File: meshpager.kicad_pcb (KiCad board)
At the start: 4 copper layers, 90 x 64 mm, 14 parts, among them J3 009155003301006, J4 USB_C_Receptacle_USB2.0_16P, J5 S8B-PH-SM4-TB, U1 RAK4630-8-SM-I

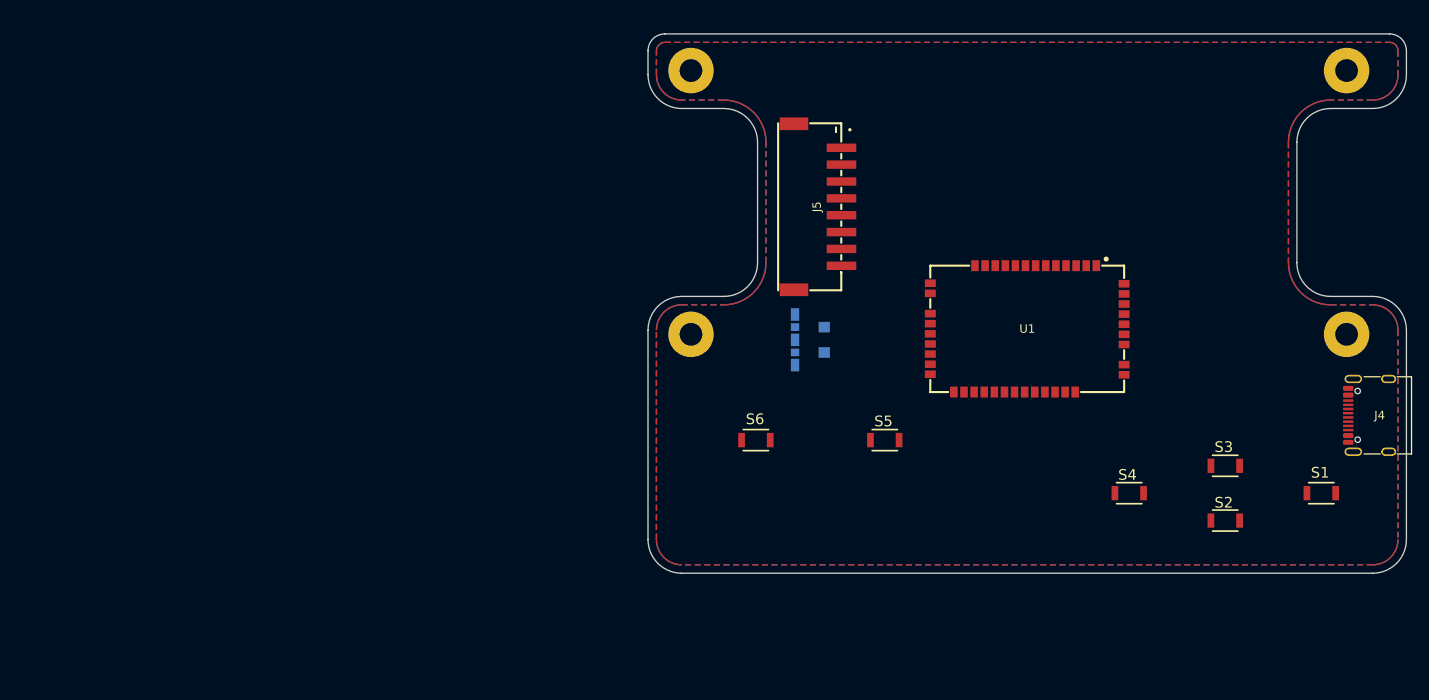
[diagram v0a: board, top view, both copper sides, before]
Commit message: Update
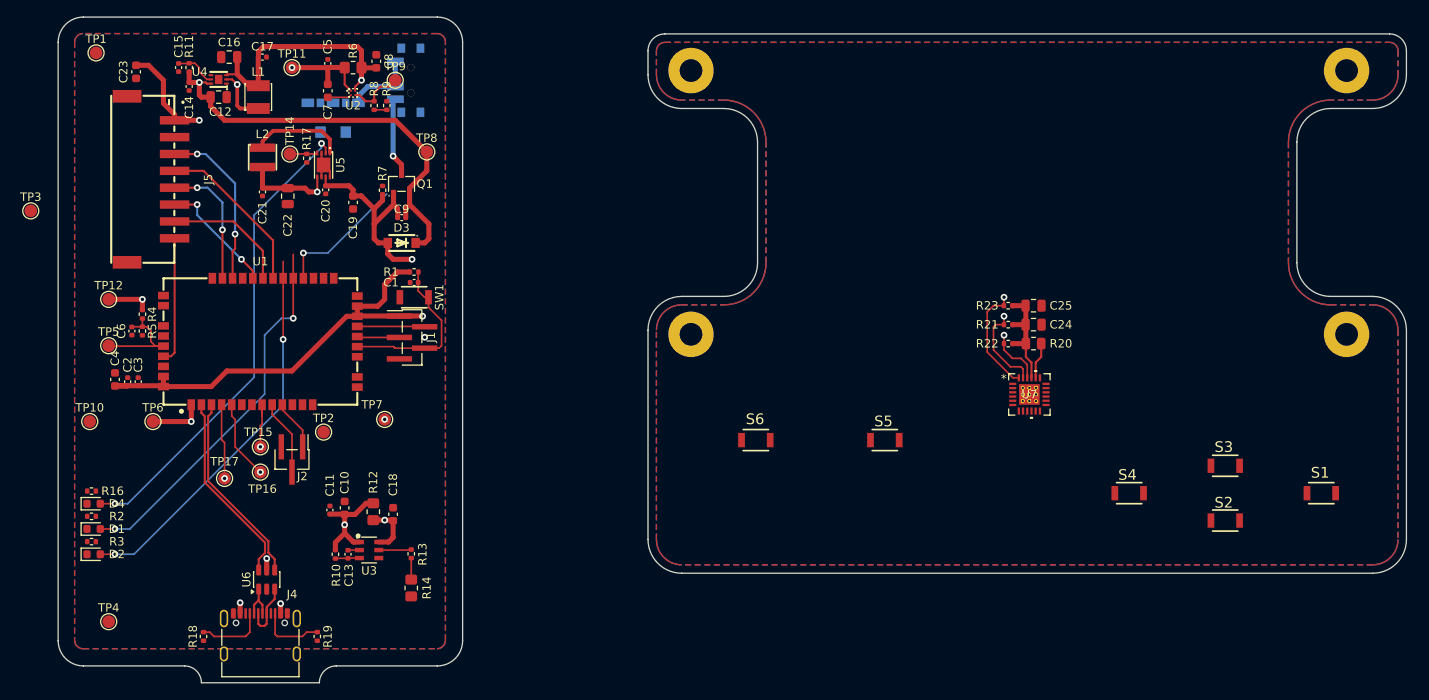
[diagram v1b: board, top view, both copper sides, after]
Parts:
- added C1: 100nF, Capacitor_SMD:C_0402_1005Metric, F.Cu at (72.2, 79.5)
- added C10: 10uF, Capacitor_SMD:C_0603_1608Metric, F.Cu at (64.0, 106.2)
- added C11: 100nF, Capacitor_SMD:C_0402_1005Metric, F.Cu at (62.2, 106.5)
- added C12: 22uF, Capacitor_SMD:C_0805_2012Metric, F.Cu at (49.0, 57.5)
- added C13: 100nF, Capacitor_SMD:C_0402_1005Metric, F.Cu at (64.4, 111.8)
- added C14: 100nF, Capacitor_SMD:C_0402_1005Metric, F.Cu at (45.5, 56.2)
- added C15: 100nF, Capacitor_SMD:C_0402_1005Metric, F.Cu at (44.3, 54.0)
- added C16: 22uF, Capacitor_SMD:C_0805_2012Metric, F.Cu at (50.3, 52.8)
- added C17: 100nF, Capacitor_SMD:C_0402_1005Metric, F.Cu at (54.2, 52.8)
- added C18: 10uF, Capacitor_SMD:C_0603_1608Metric, F.Cu at (69.8, 107.0)
- added C19: 10uF, Capacitor_SMD:C_0603_1608Metric, F.Cu at (65.0, 70.0)
- added C2: 100nF, Capacitor_SMD:C_0402_1005Metric, F.Cu at (38.2, 91.3)
- added C20: 100nF, Capacitor_SMD:C_0402_1005Metric, F.Cu at (61.8, 68.5)
- added C21: 100nF, Capacitor_SMD:C_0402_1005Metric, F.Cu at (54.2, 68.8)
- added C22: 22uF, Capacitor_SMD:C_0805_2012Metric, F.Cu at (57.2, 69.2)
- added C23: 10uF, Capacitor_SMD:C_0603_1608Metric, F.Cu at (39.2, 54.5)
- added C24: 100nF, Capacitor_SMD:C_0805_2012Metric, F.Cu at (145.8, 84.5)
- added C25: 1uF, Capacitor_SMD:C_0805_2012Metric, F.Cu at (145.8, 82.2)
- added C3: 100nF, Capacitor_SMD:C_0402_1005Metric, F.Cu at (39.5, 91.3)
- added C4: 10uF, Capacitor_SMD:C_0603_1608Metric, F.Cu at (36.8, 91.0)
- added C5: 100nF, Capacitor_SMD:C_0402_1005Metric, F.Cu at (62.0, 53.5)
- added C6: 100nF, Capacitor_SMD:C_0402_1005Metric, F.Cu at (38.8, 85.3)
- added C7: 10uF, Capacitor_SMD:C_0603_1608Metric, F.Cu at (62.0, 56.8)
- added C8: 1uF, Capacitor_SMD:C_0603_1608Metric, F.Cu at (67.8, 53.2)
- added C9: 100nF, Capacitor_SMD:C_0402_1005Metric, F.Cu at (70.8, 71.8)
- added D1: LED, LED_SMD:LED_0603_1608Metric, F.Cu at (34.2, 108.8)
- added D2: LED, LED_SMD:LED_0603_1608Metric, F.Cu at (34.2, 111.8)
- added D3: MBR140SFT1G, pager-jlc:SOD-123F_L2.8-W1.8-LS3.7-RD, F.Cu at (70.8, 74.8)
- added D4: RED, LED_SMD:LED_0603_1608Metric, F.Cu at (34.2, 105.8)
- added J1: Conn_01x05, Connector_PinHeader_1.27mm:PinHeader_1x05_P1.27mm_Vertical_SMD_Pin1Left, F.Cu at (72.0, 86.0)
- added J2: Conn_01x03, Connector_PinHeader_1.27mm:PinHeader_1x03_P1.27mm_Vertical_SMD_Pin1Left, F.Cu at (57.8, 100.5)
- added L1: 4.7uH, pager-jlc:IND-SMD_L3.0-W3.0_FNR30XXS, F.Cu at (53.8, 57.5)
- added L2: 2.2uH, pager-jlc:IND-SMD_L3.0-W3.0_SWPA3010S, F.Cu at (54.2, 64.7)
- added Q1: NCE40P05Y, pager-jlc:SOT-23-3_L2.9-W1.6-P1.90-LS2.8-BR, F.Cu at (70.8, 67.8)
- added R1: 10K, Resistor_SMD:R_0402_1005Metric, F.Cu at (72.2, 78.2)
- added R10: 100K, Resistor_SMD:R_0402_1005Metric, F.Cu at (62.9, 111.8)
- added R11: 100K, Resistor_SMD:R_0402_1005Metric, F.Cu at (45.5, 54.0)
- added R12: 0, Resistor_SMD:R_0805_2012Metric_Pad1.20x1.40mm_HandSolder, F.Cu at (67.4, 106.7)
- added R13: 470 1%, Resistor_SMD:R_0402_1005Metric, F.Cu at (71.9, 111.7)
- added R14: 0, Resistor_SMD:R_0805_2012Metric_Pad1.20x1.40mm_HandSolder, F.Cu at (71.9, 115.8)
- added R16: 1K, Resistor_SMD:R_0402_1005Metric, F.Cu at (34.0, 104.2)
- added R17: 27K, Resistor_SMD:R_0402_1005Metric, F.Cu at (59.5, 64.8)
- added R18: 5.1K, Resistor_SMD:R_0402_1005Metric, F.Cu at (47.2, 121.5)
- added R19: 5.1K, Resistor_SMD:R_0402_1005Metric, F.Cu at (60.8, 121.5)
- added R2: 1K, Resistor_SMD:R_0402_1005Metric, F.Cu at (34.0, 107.2)
- added R20: 10K, Resistor_SMD:R_0805_2012Metric, F.Cu at (145.8, 86.8)
- added R21: 10K, Resistor_SMD:R_0402_1005Metric, F.Cu at (142.8, 84.5)
- added R22: 10K, Resistor_SMD:R_0402_1005Metric, F.Cu at (142.8, 86.8)
- added R23: 10K, Resistor_SMD:R_0402_1005Metric, F.Cu at (142.7, 82.2)
- added R3: 1K, Resistor_SMD:R_0402_1005Metric, F.Cu at (34.0, 110.2)
- added R4: 1M, Resistor_SMD:R_0402_1005Metric, F.Cu at (40.0, 83.3)
- added R5: 1.5M, Resistor_SMD:R_0402_1005Metric, F.Cu at (40.0, 85.3)
- added R6: 0, Resistor_SMD:R_0805_2012Metric_Pad1.20x1.40mm_HandSolder, F.Cu at (65.0, 54.0)
- added R7: 4.7K, Resistor_SMD:R_0402_1005Metric, F.Cu at (68.5, 68.5)
- added R8: 10K, Resistor_SMD:R_0402_1005Metric, F.Cu at (67.5, 58.5)
- added R9: 100K, Resistor_SMD:R_0402_1005Metric, F.Cu at (69.0, 58.5)
- added SW1: SW_SPST, pager:B3U-1000P, F.Cu at (72.2, 81.2)
- added SW2: MK-12C02-G020, pager-jlc:SW-SMD_MK-12C02-G020, B.Cu at (71.5, 55.5)
- added TP1: GND, TestPoint:TestPoint_Pad_D1.5mm, F.Cu at (34.5, 52.2)
- added TP10: +3V3, TestPoint:TestPoint_Pad_D1.5mm, F.Cu at (33.8, 96.0)
- added TP11: +3V3_S, TestPoint:TestPoint_Pad_D1.5mm, F.Cu at (57.8, 54.0)
- added TP12: +BATT, TestPoint:TestPoint_Pad_D1.5mm, F.Cu at (36.0, 81.5)
- added TP14: CC, TestPoint:TestPoint_Pad_D1.5mm, F.Cu at (57.5, 64.2)
- added TP15: TCA_KP_INT, TestPoint:TestPoint_Pad_D1.5mm, F.Cu at (54.0, 99.0)
- added TP16: TCA_SCL, TestPoint:TestPoint_Pad_D1.5mm, F.Cu at (54.0, 102.0)
- added TP17: TCA_SDA, TestPoint:TestPoint_Pad_D1.5mm, F.Cu at (49.8, 102.8)
- added TP2: GND, TestPoint:TestPoint_Pad_D1.5mm, F.Cu at (61.5, 97.2)
- added TP3: GND, TestPoint:TestPoint_Pad_D1.5mm, F.Cu at (26.8, 71.0)
- added TP4: GND, TestPoint:TestPoint_Pad_D1.5mm, F.Cu at (36.0, 119.8)
- added TP5: VBAT_ADC, TestPoint:TestPoint_Pad_D1.5mm, F.Cu at (36.0, 87.0)
- added TP6: VBUS, TestPoint:TestPoint_Pad_D1.5mm, F.Cu at (41.2, 96.0)
- added TP7: +5V, TestPoint:TestPoint_Pad_D1.5mm, F.Cu at (68.8, 95.8)
- added TP8: VDC, TestPoint:TestPoint_Pad_D1.5mm, F.Cu at (73.8, 64.0)
- added TP9: MCU_GATE, TestPoint:TestPoint_Pad_D1.5mm, F.Cu at (70.0, 55.5)
- added U2: SGM2578AADYG/TR, pager-jlc:WLCSP-4_L0.9-W0.9-R2-C2-P0.50-TL, F.Cu at (65.0, 57.0)
- added U3: SY6287CABC, pager-jlc:SOT-23-6_L2.9-W1.6-P0.95-LS2.9-BL, F.Cu at (66.9, 111.2)
- added U4: SGM6036-3.3YUDT6G/TR, pager-jlc:UTDFN-6_L2.0-W1.5-P0.50-BL-EP, F.Cu at (49.0, 55.4)
- added U5: SGM41524YTDC8G/TR, pager-jlc:DFN-8_L3.0-W2.0-P0.50-TL-EP-1, F.Cu at (61.5, 65.5)
- added U6: USBLC6-2SC6, Package_TO_SOT_SMD:SOT-23-6, F.Cu at (54.8, 114.8)
- added U7: TCA8418RTWR, pager:RTW24_2P45X2P45, F.Cu at (145.3, 92.8)
- moved J4 135.6 mm to (54.0, 122.5), turned to 0 degrees
- moved U1 91.0 mm to (54.0, 86.5), turned to 180 degrees
- moved J5 79.2 mm to (41.0, 67.2)
- moved J3 62.4 mm to (62.6, 60.0), turned to 0 degrees
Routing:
- net +3V3: track 0.00 -> 114.7 mm, vias 0 -> 2
- net VBUS: track 0.00 -> 80.1 mm, vias 0 -> 5
- net +BATT: track 0.00 -> 78.5 mm, vias 0 -> 3
- net +5V: track 0.00 -> 67.7 mm, vias 0 -> 3
- net Net-(D4-A): track 0.00 -> 56.9 mm, vias 0 -> 2
- net +3V3_S: track 0.00 -> 52.8 mm, vias 0 -> 2
- net VDC: track 0.00 -> 51.5 mm, vias 0 -> 1
- net Net-(D2-A): track 0.00 -> 46.2 mm, vias 0 -> 2
- net Net-(D1-A): track 0.00 -> 45.0 mm, vias 0 -> 2
- net /mcu/USB_P: track 0.00 -> 23.1 mm
- net /mcu/USB_N: track 0.00 -> 23.1 mm
- net /mcu/NRF_RESET: track 0.00 -> 20.4 mm
- net /edp/EPD.MOSI: track 0.00 -> 20.0 mm, vias 0 -> 2
- net /input_module/TCA_SCL: track 0.00 -> 20.0 mm, vias 0 -> 2
- net /edp/EPD.SCK: track 0.00 -> 19.6 mm
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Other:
- board size 90 x 64 mm -> 160 x 79 mm
- board text added: "LEDS/SW"
